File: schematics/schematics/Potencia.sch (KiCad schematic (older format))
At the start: 6 parts, among them J4 Conn_01x02, U4 MT3608_PCB, U5 AMS1117

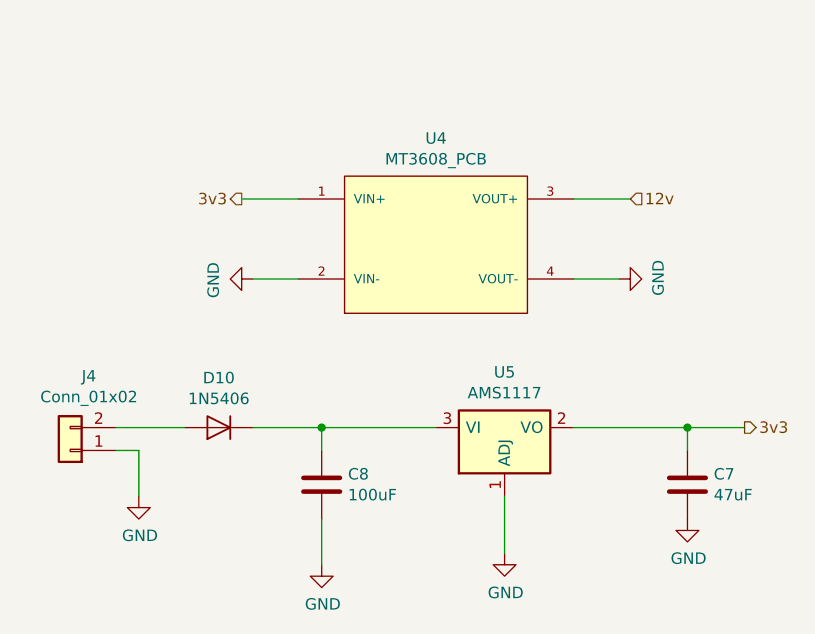
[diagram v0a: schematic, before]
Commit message: .
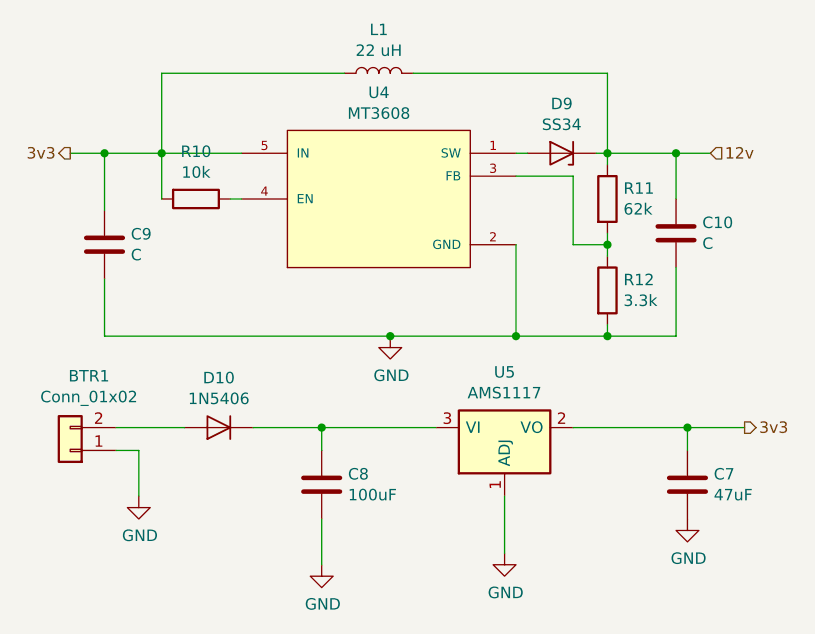
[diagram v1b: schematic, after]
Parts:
- removed U4: MT3608_PCB, mt3608:mt3608pcb, symbol MT3608:MT3608_PCB
- added C10, C9: C, Capacitor_SMD:C_0603_1608Metric_Pad1.05x0.95mm_HandSolder, symbol Device:C
- added D9: SS34, Diode_SMD:D_1206_3216Metric_Pad1.42x1.75mm_HandSolder, symbol Device:D_Zener
- added L1: 22 uH, inductor:IND_RLS-226-R, symbol Device:L
- added R10: 10k, Resistor_SMD:R_1206_3216Metric_Pad1.42x1.75mm_HandSolder, symbol Device:R
- added R11: 62k, Resistor_SMD:R_1206_3216Metric_Pad1.42x1.75mm_HandSolder, symbol Device:R
- added R12: 3.3k, Resistor_SMD:R_1206_3216Metric_Pad1.42x1.75mm_HandSolder, symbol Device:R
- added U4: MT3608, mt3608:mt3608, symbol MT3608:MT3608
- renumbered J4 to BTR1
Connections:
- net 12v: now also C10.1, D9.1 (K), L1.2, R11.1
- net 3v3: now also C9.2, L1.1, R10.2, U4.5 (IN)
- net GND: now also C10.2, C9.1, R12.2, U4.2 (GND)
- new net: D9.2 (A), U4.1 (SW)
- new net: R11.2, R12.1, U4.3 (FB)
- new net: R10.1, U4.4 (EN)
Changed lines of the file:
@@
 	4000 5350 4300 5350
 $Comp
-L Connector_Generic:Conn_01x02 J4
+L Connector_Generic:Conn_01x02 BTR1
 U 1 1 61B0FEFC
 P 3800 5450
-F 0 "J4" H 3718 5125 50  0000 C CNN
+F 0 "BTR1" H 3718 5125 50  0000 C CNN
 F 1 "Conn_01x02" H 3718 5216 50  0000 C CNN
 F 2 "Connector_JST:JST_EH_B2B-EH-A_1x02_P2.50mm_Vertical" H 3800 5450 50  0001 C CNN
@@
 Wire Wire Line
 	4000 5450 4100 5450
-$Comp
-L MT3608:MT3608_PCB U4
-U 1 1 61B2B52B
-P 5400 4550
-F 0 "U4" H 5400 5015 50  0000 C CNN
-F 1 "MT3608_PCB" H 5400 4924 50  0000 C CNN
-F 2 "mt3608:mt3608pcb" H 5050 5000 50  0001 L BNN
-F 3 "" H 5400 4550 50  0001 L BNN
-	1    5400 4550
-	1    0    0    -1
-$EndComp
-Text HLabel 4550 4350 0    50   Output ~ 0
+Text HLabel 3800 4150 0    50   Output ~ 0
 3v3
-Wire Wire Line
-	4550 4350 4800 4350
+Text HLabel 6600 4150 2    50   Input ~ 0
+12v
+$Comp
+L MT3608:MT3608 U4
+U 1 1 61B99D82
+P 5150 4350
+F 0 "U4" H 5150 4815 50  0000 C CNN
+F 1 "MT3608" H 5150 4724 50  0000 C CNN
+F 2 "mt3608:mt3608" H 5150 4350 50  0001 L BNN
+F 3 "" H 5150 4350 50  0001 L BNN
+F 4 "IPC-7351B" H 5150 4350 50  0001 L BNN "STANDARD"
+F 5 "Aero Semi" H 5150 4350 50  0001 L BNN "MANUFACTURER"
+F 6 "1.45mm" H 5150 4350 50  0001 L BNN "MAXIMUM_PACKAGE_HEIGHT"
+F 7 "1.0" H 5150 4350 50  0001 L BNN "PARTREV"
+	1    5150 4350
+	1    0    0    -1
+$EndComp
+$Comp
+L Device:L L1
+U 1 1 61B9EDF4
+P 5150 3800
+F 0 "L1" V 5340 3800 50  0000 C CNN
+F 1 "22 uH" V 5249 3800 50  0000 C CNN
+F 2 "inductor:IND_RLS-226-R" H 5150 3800 50  0001 C CNN
+F 3 "~" H 5150 3800 50  0001 C CNN
+	1    5150 3800
+	0    -1   -1   0
+$EndComp
+$Comp
+L Device:R R10
+U 1 1 61B9F732
+P 4350 4350
+F 0 "R10" V 4143 4350 50  0000 C CNN
+F 1 "10k" V 4234 4350 50  0000 C CNN
+F 2 "Resistor_SMD:R_1206_3216Metric_Pad1.42x1.75mm_HandSolder" V 4280 4350 50  0001 C CNN
+F 3 "~" H 4350 4350 50  0001 C CNN
+	1    4350 4350
+	0    1    1    0
+$EndComp
+$Comp
+L Device:R R11
+U 1 1 61BA3122
+P 6150 4350
+F 0 "R11" H 6220 4396 50  0000 L CNN
+F 1 "62k" H 6220 4305 50  0000 L CNN
+F 2 "Resistor_SMD:R_1206_3216Metric_Pad1.42x1.75mm_HandSolder" V 6080 4350 50  0001 C CNN
+F 3 "~" H 6150 4350 50  0001 C CNN
+	1    6150 4350
+	1    0    0    -1
+$EndComp
+$Comp
+L Device:R R12
+U 1 1 61BA3451
+P 6150 4750
+F 0 "R12" H 6220 4796 50  0000 L CNN
+F 1 "3.3k" H 6220 4705 50  0000 L CNN
+F 2 "Resistor_SMD:R_1206_3216Metric_Pad1.42x1.75mm_HandSolder" V 6080 4750 50  0001 C CNN
+F 3 "~" H 6150 4750 50  0001 C CNN
+	1    6150 4750
+	1    0    0    -1
+$EndComp
+$Comp
+L Device:C C10
+U 1 1 61BA3A9C
+P 6450 4500
+F 0 "C10" H 6565 4546 50  0000 L CNN
+F 1 "C" H 6565 4455 50  0000 L CNN
+F 2 "Capacitor_SMD:C_0603_1608Metric_Pad1.05x0.95mm_HandSolder" H 6488 4350 50  0001 C CNN
+F 3 "~" H 6450 4500 50  0001 C CNN
+	1    6450 4500
+	1    0    0    -1
+$EndComp
+Wire Wire Line
+	4500 4350 4550 4350
+Wire Wire Line
+	4200 4350 4200 4150
+Wire Wire Line
+	4200 4150 3950 4150
+Wire Wire Line
+	4200 4150 4550 4150
+Connection ~ 4200 4150
+Connection ~ 3950 4150
+Wire Wire Line
+	3950 4150 3800 4150
+Wire Wire Line
+	4200 4150 4200 3800
+Wire Wire Line
+	4200 3800 5000 3800
+$Comp
+L Device:D_Zener D9
+U 1 1 61BAC067
+P 5950 4150
+F 0 "D9" H 5950 3934 50  0000 C CNN
+F 1 "SS34" H 5950 4025 50  0000 C CNN
+F 2 "Diode_SMD:D_1206_3216Metric_Pad1.42x1.75mm_HandSolder" H 5950 4150 50  0001 C CNN
+F 3 "~" H 5950 4150 50  0001 C CNN
+	1    5950 4150
+	-1   0    0    1
+$EndComp
+Wire Wire Line
+	6150 4200 6150 4150
+Wire Wire Line
+	6100 4150 6150 4150
+Connection ~ 6150 4150
+Wire Wire Line
+	5800 4150 5750 4150
+Wire Wire Line
+	5300 3800 6150 3800
+Wire Wire Line
+	6150 3800 6150 4150
+Wire Wire Line
+	6150 4500 6150 4550
+Wire Wire Line
+	6150 4550 6000 4550
+Wire Wire Line
+	6000 4550 6000 4250
+Wire Wire Line
+	6000 4250 5750 4250
+Connection ~ 6150 4550
+Wire Wire Line
+	6150 4550 6150 4600
+Wire Wire Line
+	6150 4150 6450 4150
+Wire Wire Line
+	6450 4150 6450 4350
+Connection ~ 6450 4150
+Wire Wire Line
+	6450 4150 6600 4150
 $Comp
 L power:GND #PWR0118
-U 1 1 61B2F399
-P 4600 4700
-F 0 "#PWR0118" H 4600 4450 50  0001 C CNN
-F 1 "GND" H 4605 4527 50  0000 C CNN
-F 2 "" H 4600 4700 50  0001 C CNN
-F 3 "" H 4600 4700 50  0001 C CNN
-	1    4600 4700
-	0    1    1    0
-$EndComp
-Wire Wire Line
-	4600 4700 4800 4700
-$Comp
-L power:GND #PWR0123
-U 1 1 61B301DD
-P 6200 4700
-F 0 "#PWR0123" H 6200 4450 50  0001 C CNN
-F 1 "GND" H 6205 4527 50  0000 C CNN
-F 2 "" H 6200 4700 50  0001 C CNN
-F 3 "" H 6200 4700 50  0001 C CNN
-	1    6200 4700
-	0    -1   -1   0
-$EndComp
-Wire Wire Line
-	6200 4700 6000 4700
-Text HLabel 6250 4350 2    50   Input ~ 0
-12v
-Wire Wire Line
-	6250 4350 6000 4350
+U 1 1 61BBC041
+P 5200 4950
+F 0 "#PWR0118" H 5200 4700 50  0001 C CNN
+F 1 "GND" H 5205 4777 50  0000 C CNN
+F 2 "" H 5200 4950 50  0001 C CNN
+F 3 "" H 5200 4950 50  0001 C CNN
+	1    5200 4950
+	1    0    0    -1
+$EndComp
+Wire Wire Line
+	5200 4950 5750 4950
+Wire Wire Line
+	6150 4950 6150 4900
+Wire Wire Line
+	6150 4950 6450 4950
+Wire Wire Line
+	6450 4950 6450 4650
+Connection ~ 6150 4950
+Wire Wire Line
+	5750 4550 5750 4950
+Connection ~ 5750 4950
+Wire Wire Line
+	5750 4950 6150 4950
+Wire Wire Line
+	5200 4950 3950 4950
+Wire Wire Line
+	3950 4950 3950 4700
+Connection ~ 5200 4950
+$Comp
+L Device:C C9
+U 1 1 61BA1FAF
+P 3950 4550
+F 0 "C9" H 3835 4504 50  0000 R CNN
+F 1 "C" H 3835 4595 50  0000 R CNN
+F 2 "Capacitor_SMD:C_0603_1608Metric_Pad1.05x0.95mm_HandSolder" H 3988 4400 50  0001 C CNN
+F 3 "~" H 3950 4550 50  0001 C CNN
+	1    3950 4550
+	-1   0    0    1
+$EndComp
+Wire Wire Line
+	3950 4150 3950 4400
 $EndSCHEMATC
